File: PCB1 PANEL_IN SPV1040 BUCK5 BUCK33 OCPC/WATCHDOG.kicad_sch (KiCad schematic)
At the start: 6 parts, among them SW2 KMR231NG LFS, U22 MAX706RESA

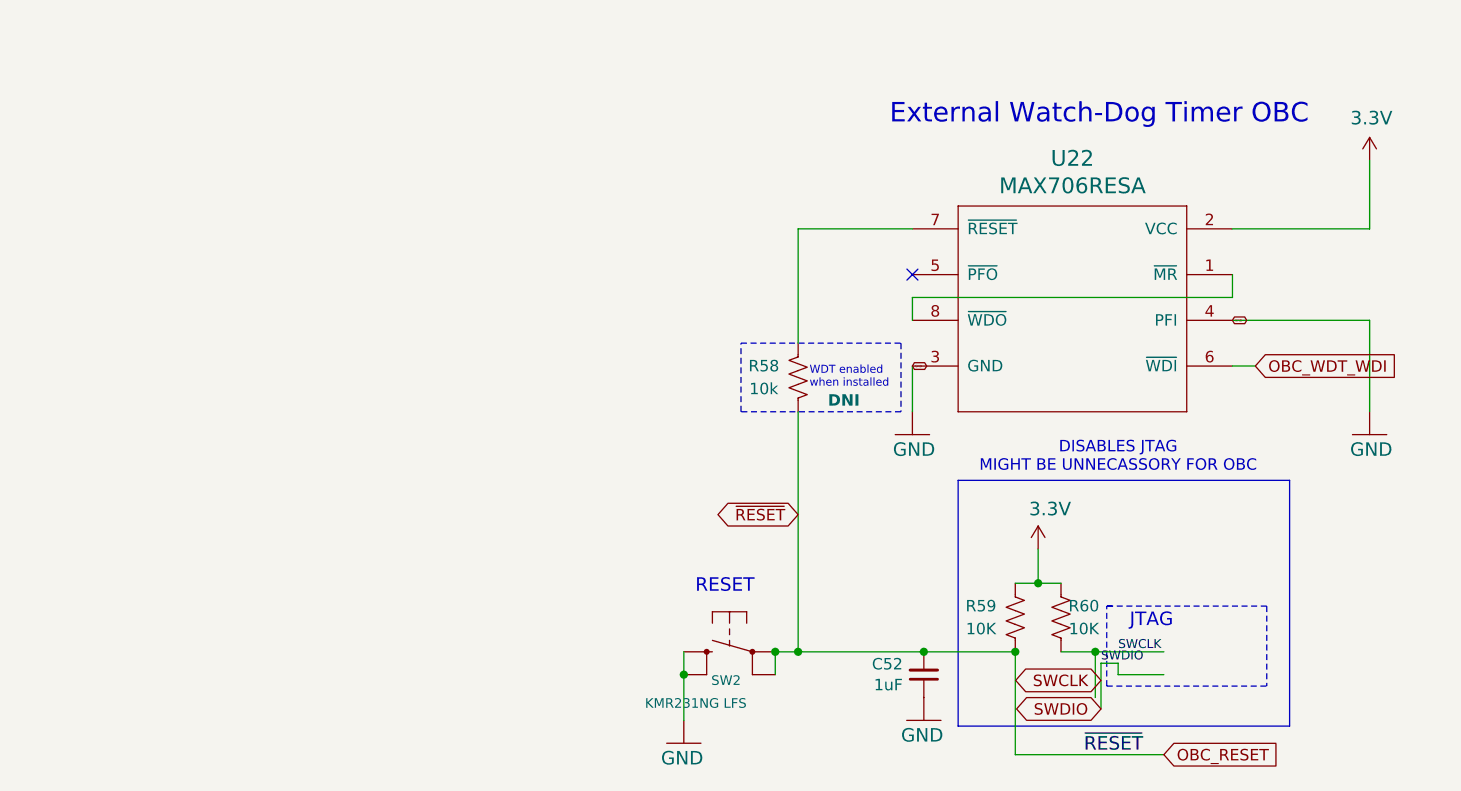
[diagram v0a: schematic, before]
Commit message: VCOMMIT
EDITS N+I
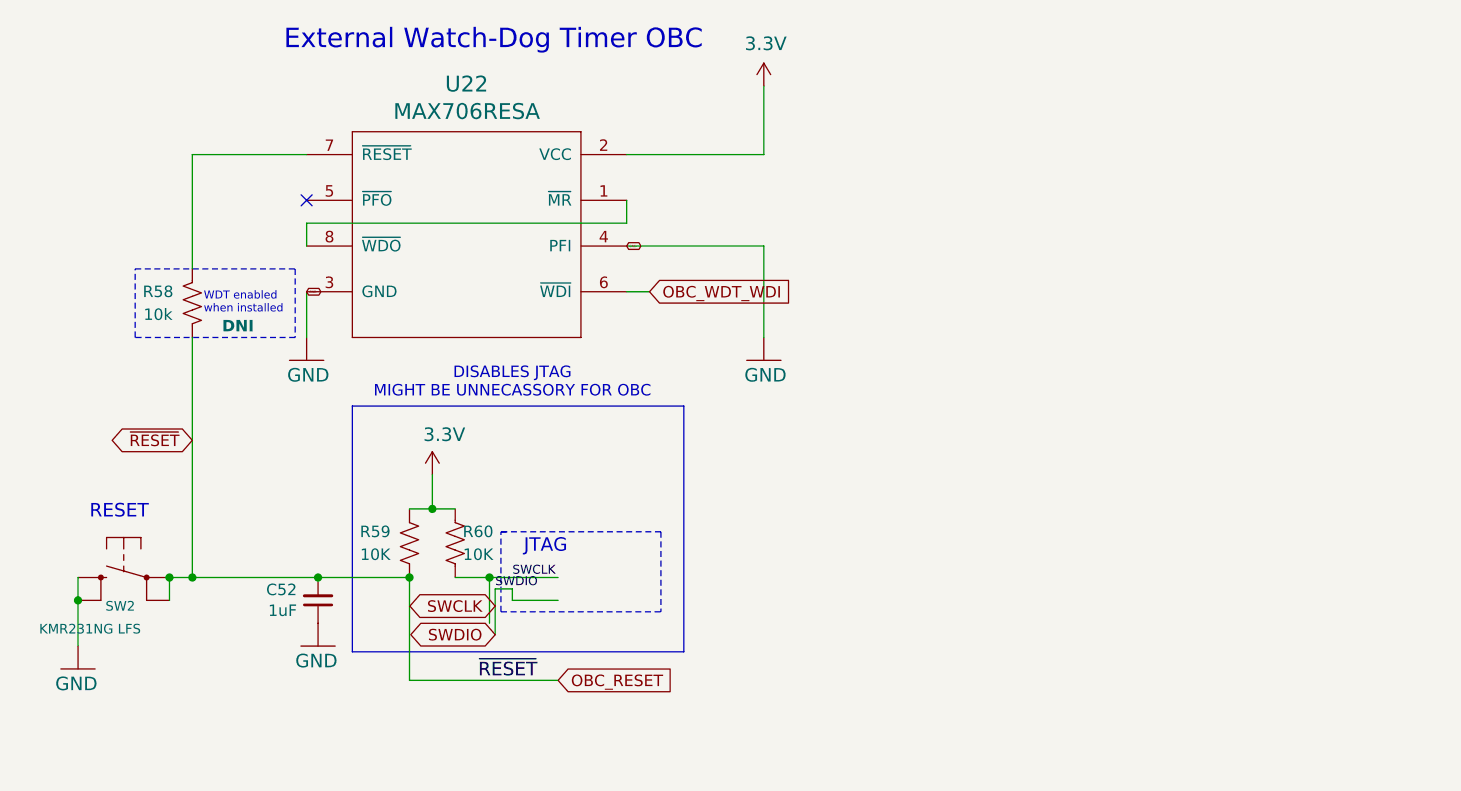
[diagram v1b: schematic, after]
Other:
- moved on the sheet: C52, R58, R59, R60, SW2, U22
